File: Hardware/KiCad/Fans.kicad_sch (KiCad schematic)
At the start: 16 parts, among them J9 Conn_01x06, Q1 IRLML0030, Q2 IRLML0030

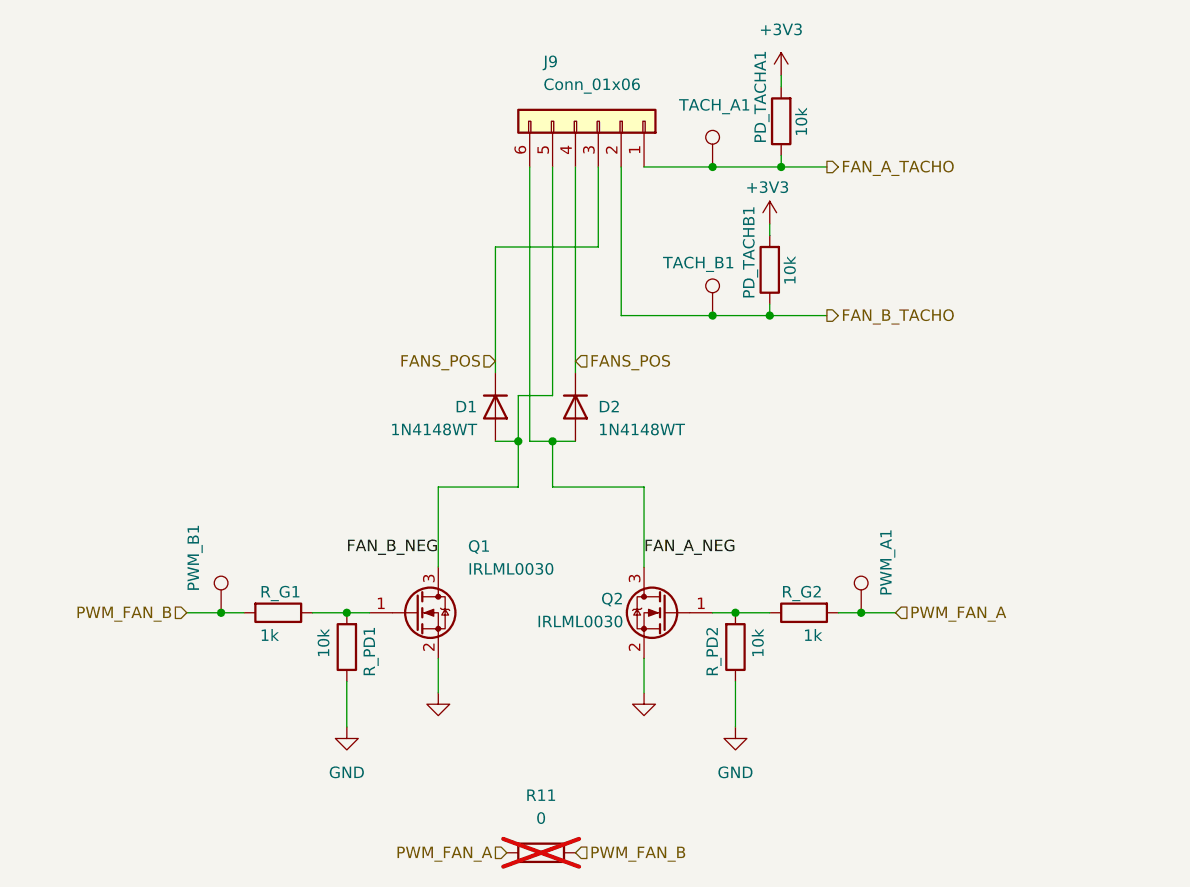
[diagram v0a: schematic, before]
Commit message: done with changes
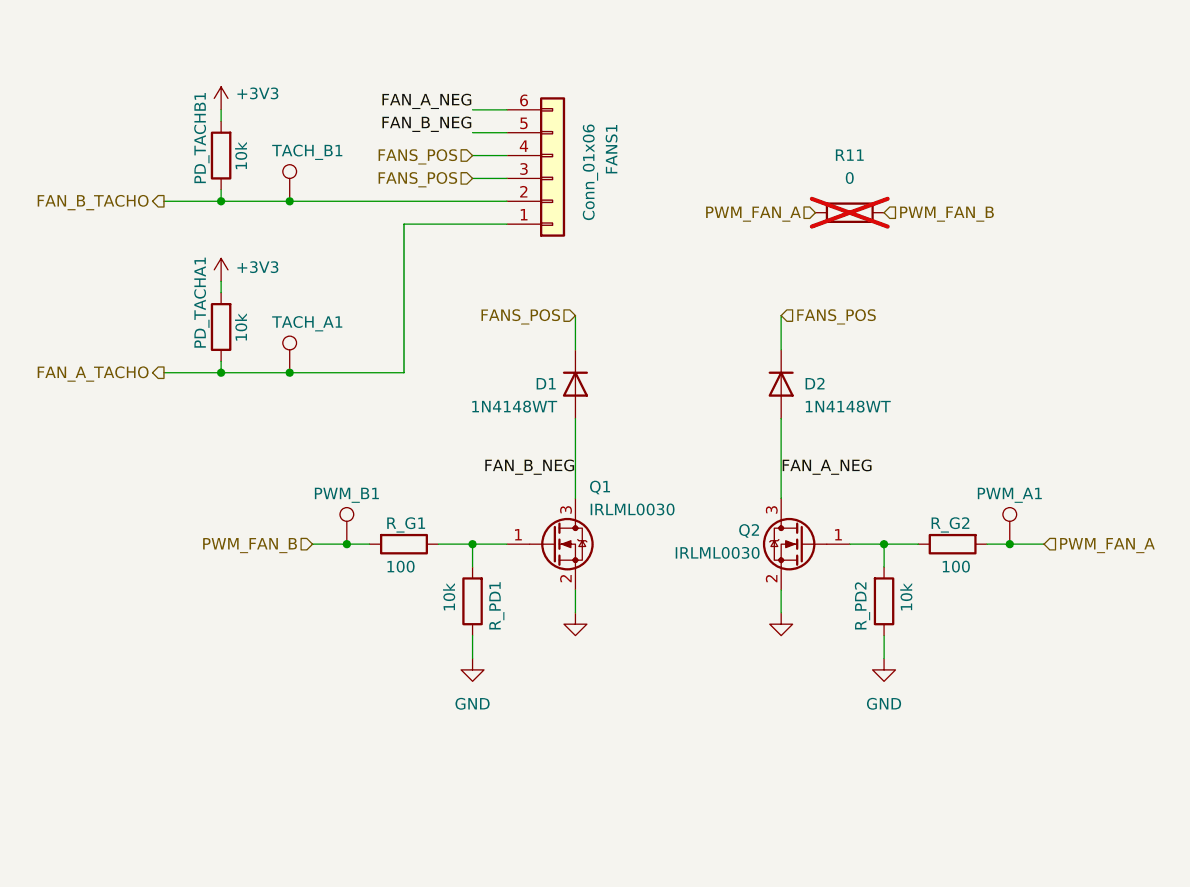
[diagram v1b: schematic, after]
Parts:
- PWM_A1, PWM_B1: footprint TestPoint:TestPoint_Pin_1.0x1.0mm -> TestPoint:TestPoint_Keystone_5000-5004_Miniature; now in the parts list
- R_G1, R_G2: value 1k -> 100
- TACH_A1, TACH_B1: footprint TestPoint:TestPoint_Pin_1.0x1.0mm -> TestPoint:TestPoint_Pad_1.0x1.0mm; now in the parts list
- renumbered J9 to FANS1
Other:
- moved on the sheet: D1, D2, FANS1, PD_TACHA1, PD_TACHB1, PWM_A1, PWM_B1, Q1, Q2, R11, R_G1, R_G2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
